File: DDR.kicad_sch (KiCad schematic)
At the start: 1 part, among them U2 rv1126/rv1109

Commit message: updated: titles
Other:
- title: Leaf RV1126 PMIC RK809 Codec -> Leaf RV1126 RK809 DDR
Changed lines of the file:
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@@
   (paper "A4")
   (title_block
-    (title "Leaf RV1126 PMIC RK809 Codec")
+    (title "Leaf RV1126 RK809 DDR")
     (date "2023-02-25")
     (rev "1")

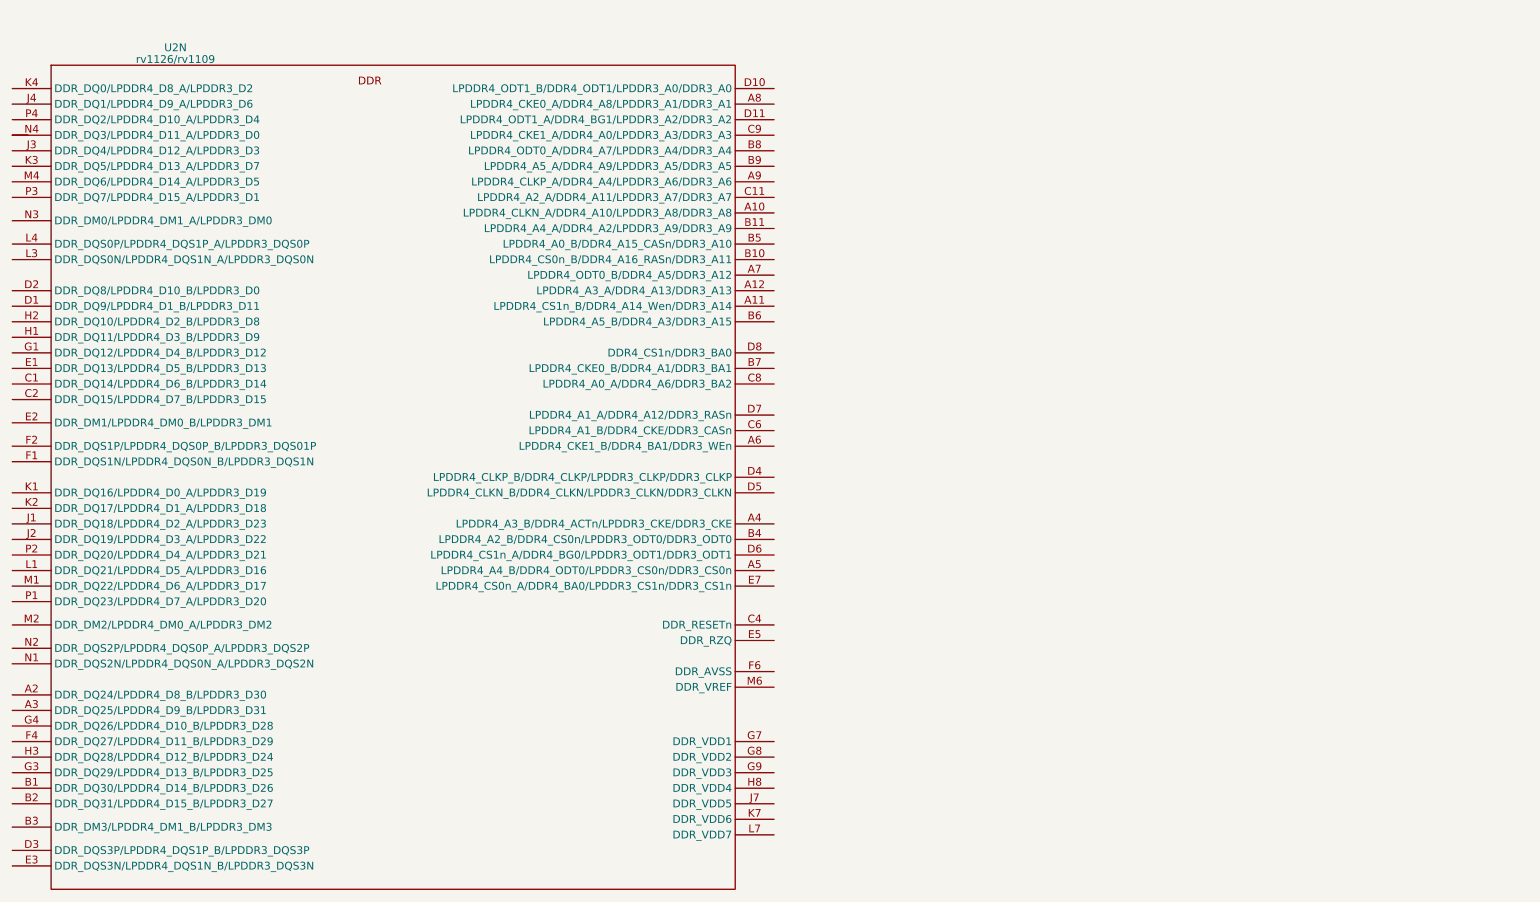
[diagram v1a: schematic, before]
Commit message: updated: DDR
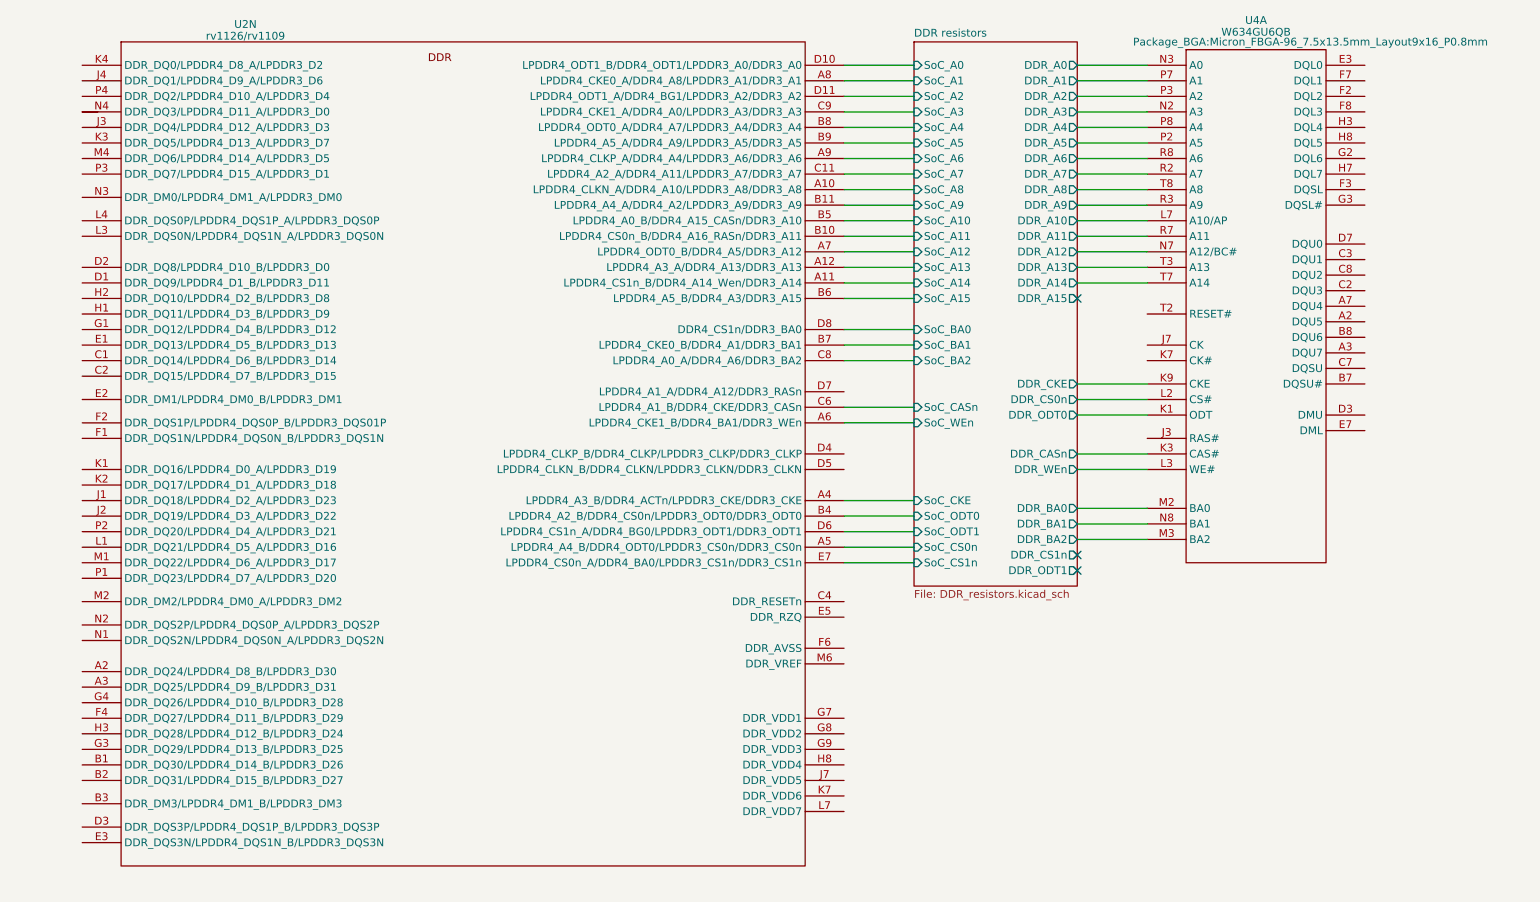
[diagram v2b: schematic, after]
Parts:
- added U4: W634GU6QB, Package_BGA:Micron_FBGA-96_7.5x13.5mm_Layout9x16_P0.8mm, symbol Memory_DDR:W634GU6QB
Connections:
- net DDR resistors/SoC_A8: now reaches U2.A10 (LPDDR4_CLKN_A/DDR4_A10/LPDDR3_A8/DDR3_A8)
- net DDR resistors/SoC_A14: now reaches U2.A11 (LPDDR4_CS1n_B/DDR4_A14_Wen/DDR3_A14)
- net DDR resistors/SoC_A13: now reaches U2.A12 (LPDDR4_A3_A/DDR4_A13/DDR3_A13)
- net DDR resistors/SoC_CKE: now reaches U2.A4 (LPDDR4_A3_B/DDR4_ACTn/LPDDR3_CKE/DDR3_CKE)
- net DDR resistors/SoC_CS0n: now reaches U2.A5 (LPDDR4_A4_B/DDR4_ODT0/LPDDR3_CS0n/DDR3_CS0n)
- net DDR resistors/SoC_WEn: now reaches U2.A6 (LPDDR4_CKE1_B/DDR4_BA1/DDR3_WEn)
- net DDR resistors/SoC_A12: now reaches U2.A7 (LPDDR4_ODT0_B/DDR4_A5/DDR3_A12)
- net DDR resistors/SoC_A1: now reaches U2.A8 (LPDDR4_CKE0_A/DDR4_A8/LPDDR3_A1/DDR3_A1)
- net DDR resistors/SoC_A6: now reaches U2.A9 (LPDDR4_CLKP_A/DDR4_A4/LPDDR3_A6/DDR3_A6)
- net DDR resistors/SoC_A11: now reaches U2.B10 (LPDDR4_CS0n_B/DDR4_A16_RASn/DDR3_A11)
- net DDR resistors/SoC_A9: now reaches U2.B11 (LPDDR4_A4_A/DDR4_A2/LPDDR3_A9/DDR3_A9)
- net DDR resistors/SoC_ODT0: now reaches U2.B4 (LPDDR4_A2_B/DDR4_CS0n/LPDDR3_ODT0/DDR3_ODT0)
- net DDR resistors/SoC_A10: now reaches U2.B5 (LPDDR4_A0_B/DDR4_A15_CASn/DDR3_A10)
- net DDR resistors/SoC_A15: now reaches U2.B6 (LPDDR4_A5_B/DDR4_A3/DDR3_A15)
- net DDR resistors/SoC_BA1: now reaches U2.B7 (LPDDR4_CKE0_B/DDR4_A1/DDR3_BA1)
- net DDR resistors/SoC_A4: now reaches U2.B8 (LPDDR4_ODT0_A/DDR4_A7/LPDDR3_A4/DDR3_A4)
- net DDR resistors/SoC_A5: now reaches U2.B9 (LPDDR4_A5_A/DDR4_A9/LPDDR3_A5/DDR3_A5)
- net DDR resistors/SoC_A7: now reaches U2.C11 (LPDDR4_A2_A/DDR4_A11/LPDDR3_A7/DDR3_A7)
- net DDR resistors/SoC_CASn: now reaches U2.C6 (LPDDR4_A1_B/DDR4_CKE/DDR3_CASn)
- net DDR resistors/SoC_BA2: now reaches U2.C8 (LPDDR4_A0_A/DDR4_A6/DDR3_BA2)
- net DDR resistors/SoC_A3: now reaches U2.C9 (LPDDR4_CKE1_A/DDR4_A0/LPDDR3_A3/DDR3_A3)
- net DDR resistors/SoC_A0: now reaches U2.D10 (LPDDR4_ODT1_B/DDR4_ODT1/LPDDR3_A0/DDR3_A0)
- net DDR resistors/SoC_A2: now reaches U2.D11 (LPDDR4_ODT1_A/DDR4_BG1/LPDDR3_A2/DDR3_A2)
- net DDR resistors/SoC_ODT1: now reaches U2.D6 (LPDDR4_CS1n_A/DDR4_BG0/LPDDR3_ODT1/DDR3_ODT1)
- net DDR resistors/SoC_BA0: now reaches U2.D8 (DDR4_CS1n/DDR3_BA0)
- net DDR resistors/SoC_CS1n: now reaches U2.E7 (LPDDR4_CS0n_A/DDR4_BA0/LPDDR3_CS1n/DDR3_CS1n)
- new net DDR resistors/DDR_A0: U4.N3 (A0)
- new net DDR resistors/DDR_A1: U4.P7 (A1)
- new net DDR resistors/DDR_A10: U4.L7 (A10/AP)
- new net DDR resistors/DDR_A11: U4.R7 (A11)
- new net DDR resistors/DDR_A12: U4.N7 (A12/BC#)
- new net DDR resistors/DDR_A13: U4.T3 (A13)
- new net DDR resistors/DDR_A14: U4.T7 (A14)
- new net DDR resistors/DDR_A2: U4.P3 (A2)
- new net DDR resistors/DDR_A3: U4.N2 (A3)
- new net DDR resistors/DDR_A4: U4.P8 (A4)
- new net DDR resistors/DDR_A5: U4.P2 (A5)
- new net DDR resistors/DDR_A6: U4.R8 (A6)
- new net DDR resistors/DDR_A7: U4.R2 (A7)
- new net DDR resistors/DDR_A8: U4.T8 (A8)
- new net DDR resistors/DDR_A9: U4.R3 (A9)
- new net DDR resistors/DDR_BA0: U4.M2 (BA0)
- new net DDR resistors/DDR_BA1: U4.N8 (BA1)
- new net DDR resistors/DDR_BA2: U4.M3 (BA2)
- new net DDR resistors/DDR_CASn: U4.K3 (CAS#)
- new net DDR resistors/DDR_CKE: U4.K9 (CKE)
- new net DDR resistors/DDR_CS0n: U4.L2 (CS#)
- new net DDR resistors/DDR_ODT0: U4.K1 (ODT)
- new net DDR resistors/DDR_WEn: U4.L3 (WE#)
- no-connect marks 0 -> 3
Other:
- added sheet DDR resistors (DDR_resistors.kicad_sch)
- moved on the sheet: U2N
